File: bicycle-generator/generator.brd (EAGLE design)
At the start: 93.7 x 69.8 mm, 62 parts, among them IC1 MC34063AD, K1 ARK500/2, K2 ARK500/2, K3 ARK500/2, K4 ARK500/2, K5 ARK500/2, K6 HEAT_NPN, K7 ARK500/2, K8 ARK500/2, Q1 IRF3704S, Q2 IRF3704S, T1 BC807, T2 BC807, X1 CV_LED, X2 PWR_LED, X3 5V_SW, X4 5V_LED, X5 5V_OUT

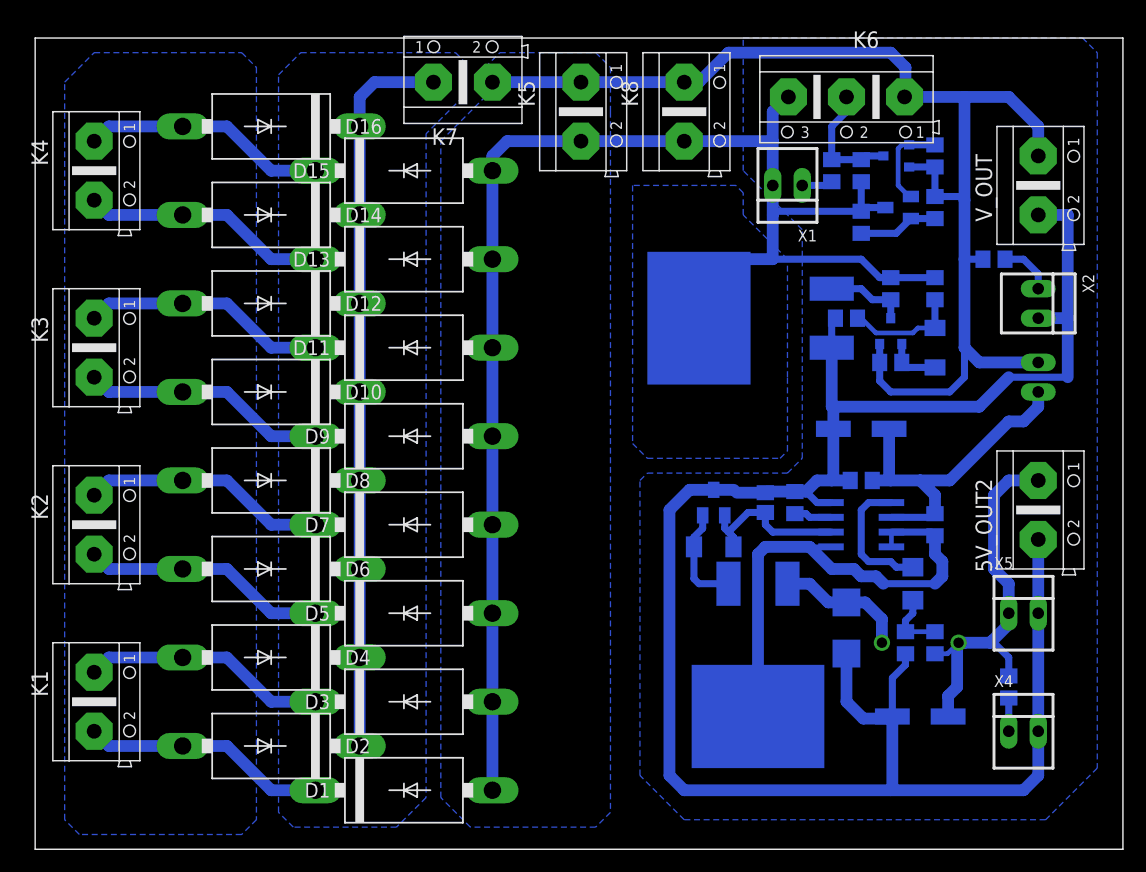
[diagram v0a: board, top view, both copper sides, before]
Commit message: Commit before merge
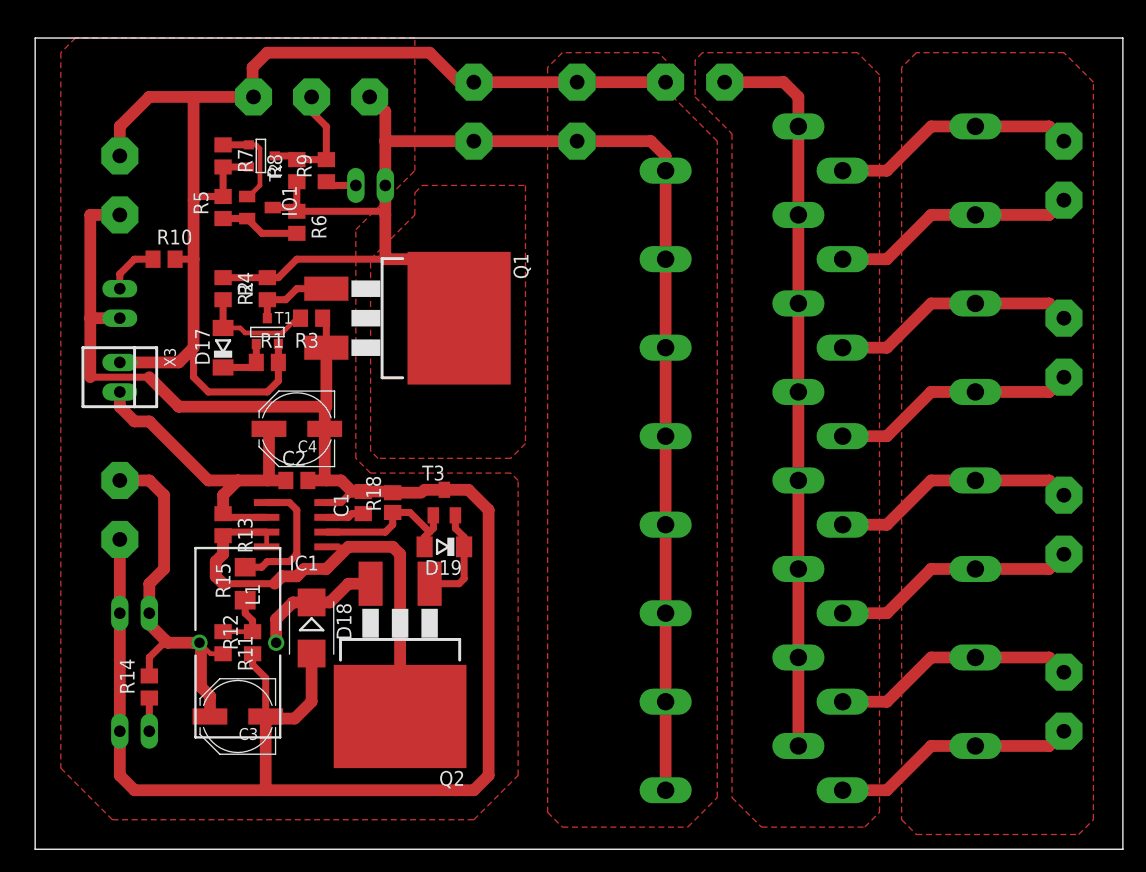
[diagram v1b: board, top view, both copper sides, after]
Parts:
- moved K1 83.5 mm to (88.6, 22.9), flipped to the bottom
- moved K2 83.5 mm to (88.6, 38.1), flipped to the bottom
- moved K3 83.5 mm to (88.6, 53.3), flipped to the bottom
- moved K4 83.5 mm to (88.6, 68.6), flipped to the bottom
- moved 5V_OUT2 79.1 mm to (7.29, 39.4), flipped to the bottom
- moved V_OUT 79.1 mm to (7.29, 67.3), flipped to the bottom
- moved X2 79.1 mm to (7.29, 57.1), flipped to the bottom
- moved X3 79.1 mm to (7.29, 50.8), flipped to the top
- moved X4 76.5 mm to (8.56, 20.3), flipped to the bottom
- moved X5 76.5 mm to (8.56, 30.5), flipped to the bottom
- moved R14 74.0 mm to (9.83, 24.1), flipped to the top
- moved R10 71.5 mm to (11.1, 61.0), flipped to the top
- moved D17 61.3 mm to (16.2, 53.3), flipped to the top
- moved R11 61.3 mm to (16.2, 27.9), flipped to the top
- moved R13 61.3 mm to (16.2, 38.1), flipped to the top
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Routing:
- added copper zone on layer 1, net GND
- added copper zone on layer 1, net N$20
- added copper zone on layer 1, net N$25
- added copper zone on layer 1, net V-
- removed copper zone on layer 16, net GND
- removed copper zone on layer 16, net N$20
- removed copper zone on layer 16, net N$25
- removed copper zone on layer 16, net V-
